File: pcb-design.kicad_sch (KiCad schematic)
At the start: 7 parts, among them J2 SM06B-SRSS-TBLFSN, U2 OS102011MA1QS1, U4 MOUDLE-SEEEDUINO-XIAO-ESP32C3

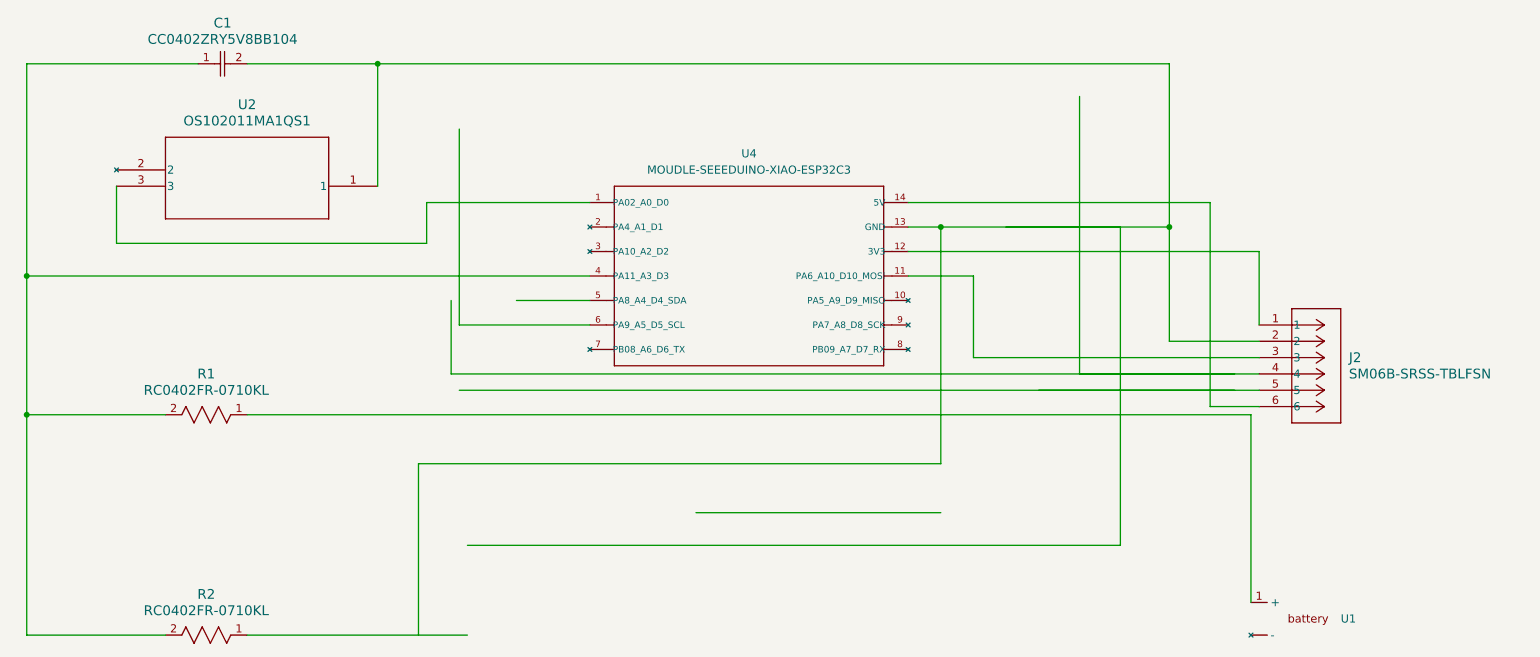
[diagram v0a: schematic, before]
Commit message: pcb fixes for 4.1
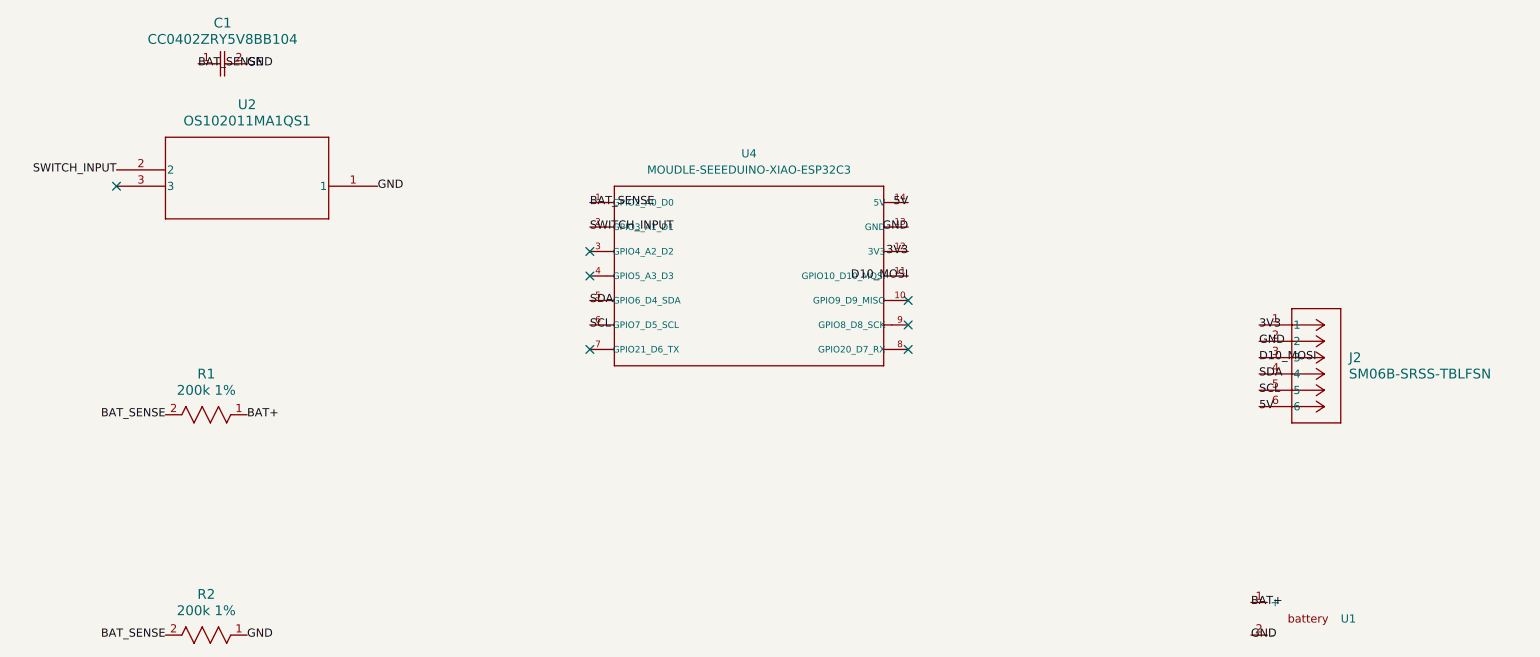
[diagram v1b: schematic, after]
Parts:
- C1: footprint YAG_CC0402_YAG -> CC0402ZRY5V8BB104:YAG_CC0402_YAG; symbol 2023-11-23_19-16-20:CC0402ZRY5V8BB104 -> CC0402ZRY5V8BB104:CC0402ZRY5V8BB104
- J2: footprint CONN_SM06B-SRSS-TB_JST -> SM06B-SRSS-TB:CONN_SM06B-SRSS-TB_JST
- R1, R2: value RC0402FR-0710KL -> 200k 1%; footprint RC0402N_YAG -> RC0402FR-0710KL:RC0402N_YAG; symbol 2023-11-23_19-25-58:RC0402FR-0710KL -> RC0402FR-0710KL:RC0402FR-0710KL
- U2: footprint SWITCH_11MA1QS1 -> OS102011MA1QS1:SWITCH_11MA1QS1; symbol 2023-11-23_19-58-11:OS102011MA1QS1 -> OS102011MA1QS1:OS102011MA1QS1
- U4: footprint MOUDLE14P-SMD-2.54-21X17.8MM -> XIAO_ESP32C3:MOUDLE14P-SMD-2.54-21X17.8MM; symbol MOUDLE-SEEEDUINO-XIAO-ESP32C3-2:MOUDLE-SEEEDUINO-XIAO-ESP32C3 -> XIAO_ESP32C3:MOUDLE-SEEEDUINO-XIAO-ESP32C3
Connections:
- net at U2.3: no longer U4.1 (PA02_A0_D0)
- net D10_MOSI: now reaches J2.3, U4.11 (GPIO10_D10_MOSI)
- net 3V3: now reaches J2.1, U4.12 (3V3)
- net GND: now reaches C1.2, J2.2, U2.1, U4.13 (GND)
- net GND: now also R2.1, U1.2 (-)
- net 5V: now reaches J2.6, U4.14 (5V)
- net SWITCH_INPUT: now reaches U4.2 (GPIO3_A1_D1)
- net SWITCH_INPUT: now also U2.2
- net BAT_SENSE: now reaches C1.1, R1.2, R2.2
- net BAT_SENSE: now also U4.1 (GPIO2_A0_D0); no longer U4.4 (PA11_A3_D3)
- net SDA: now reaches U4.5 (GPIO6_D4_SDA)
- net SDA: now also J2.4
- net SCL: now reaches U4.6 (GPIO7_D5_SCL)
- net SCL: now also J2.5
- net BAT+: now reaches R1.1, U1.1 (+)
- no-connect marks 0 -> 7
